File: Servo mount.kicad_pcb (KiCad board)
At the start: 2 copper layers, 80 x 34.1 mm, 40 parts, among them IC1 ATTINY84-SS, J1 SOLDER_PAD, J2 SOLDER_PAD, J3 SOLDER_PAD, J5 SOLDER_PAD, J6 SOLDER_PAD, J7 SOLDER_PAD, J8 SOLDER_PAD, K5 CONN_3, K6 CONN_3, P1 CONN_3X2, Q1 BC847, Q2 BC847, U1 uA78L05, U2 BUZ11

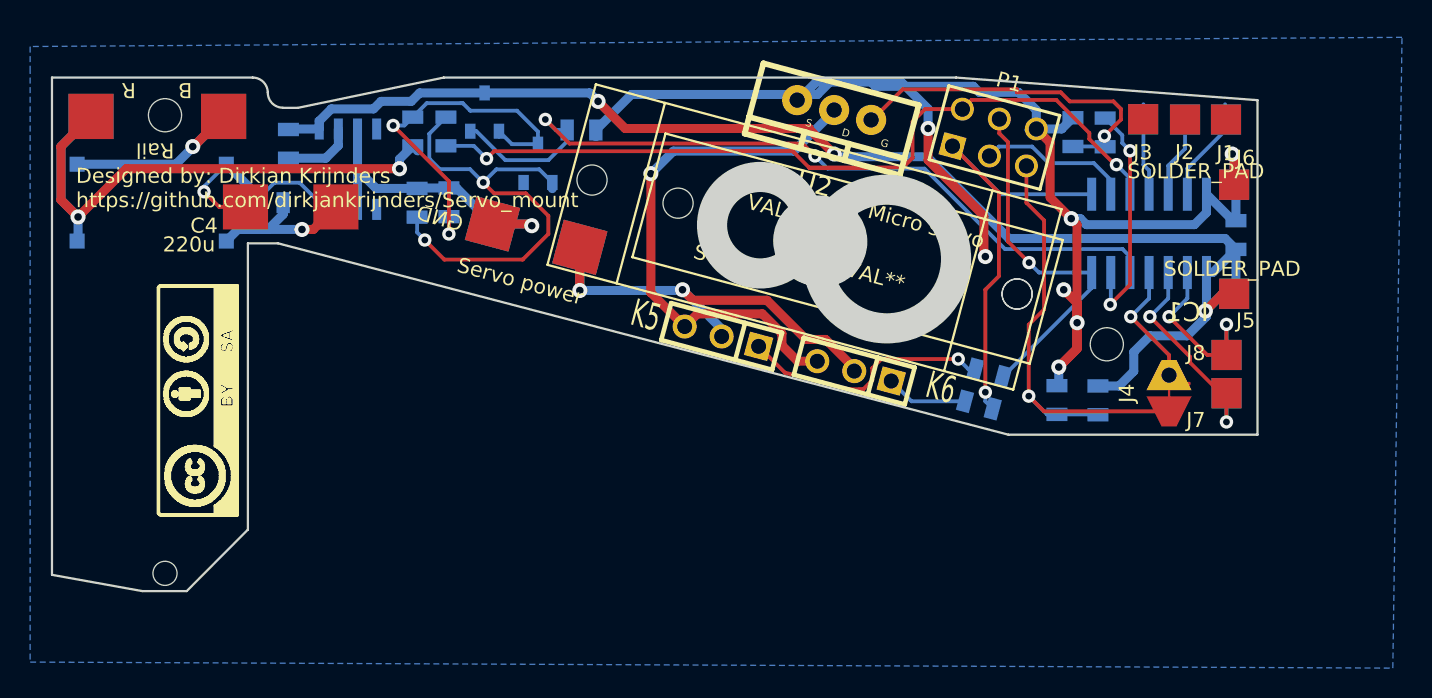
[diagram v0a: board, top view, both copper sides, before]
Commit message: Updates to rev. 3x
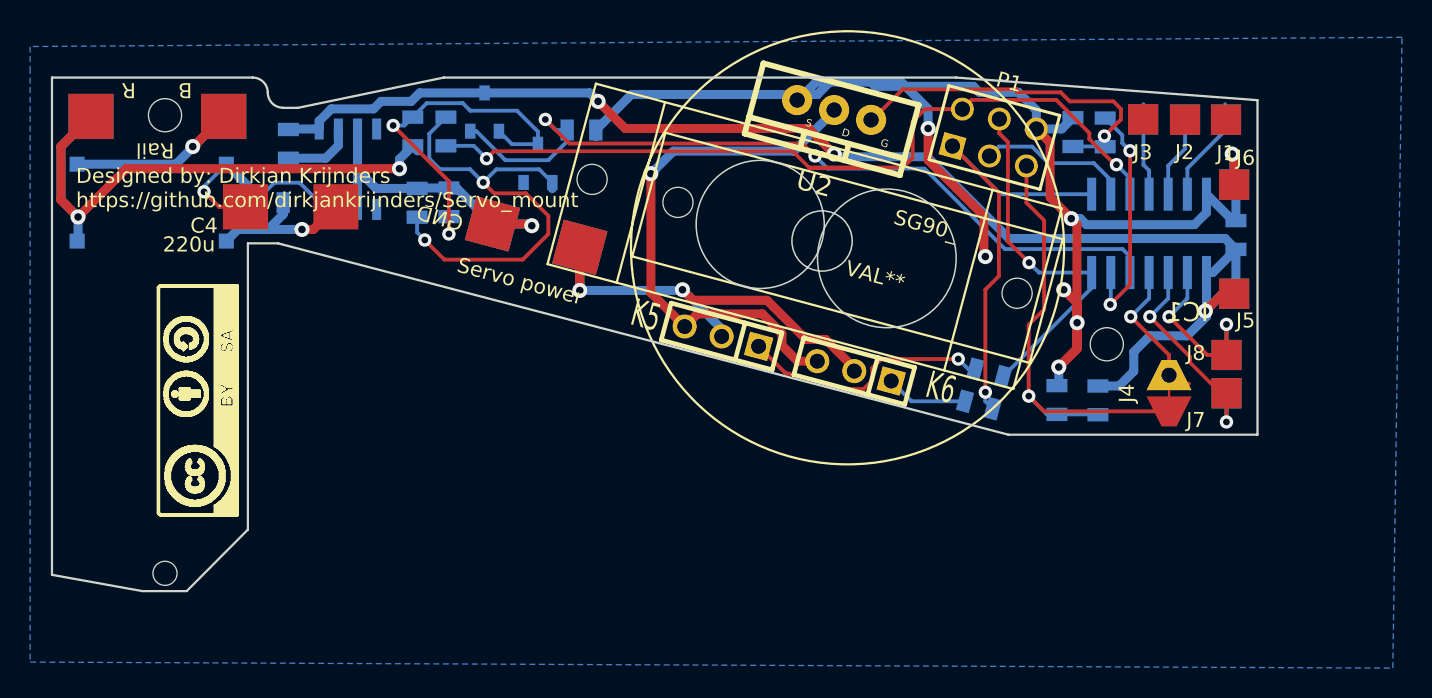
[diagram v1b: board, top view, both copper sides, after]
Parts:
- removed Micro servo: VAL**, Micro_servo
- SG90_: footprint Pyth_servos:Micro_servo_SG90 -> Pyth_servos:Combined_servo
- moved SG90_ 2.94 mm to (152.8, 111.3), turned to 345 degrees
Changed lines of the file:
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@@
     (tracks 380)
     (zones 0)
-    (modules 40)
+    (modules 39)
     (nets 26)
   )
@@
       (net 2 -VAA))
   )
-  (module Micro_servo (layer F.Cu)
-    (at 152.8 111.35 345)
-    (tags HD-1370A)
-    (fp_text reference "Micro servo" (at 4.65 -2.8 345) (layer F.SilkS)
-      (effects (font (size 1 1) (thickness 0.15)))
-    )
-    (fp_text value VAL** (at 2.25 1.3 345) (layer F.SilkS)
-      (effects (font (size 1 1) (thickness 0.15)))
-    )
-    (fp_circle (center -2 0) (end 0 -0.2) (layer Edge.Cuts) (width 2))
-    (fp_circle (center -6 0) (end -3.5 2) (layer Edge.Cuts) (width 2))
-    (fp_line (start 13.65 4.25) (end -13.65 4.25) (layer F.SilkS) (width 0.15))
-    (fp_line (start -13.65 -4.25) (end 13.65 -4.25) (layer F.SilkS) (width 0.15))
-    (fp_line (start 13.65 -4.25) (end 13.65 4.25) (layer F.SilkS) (width 0.15))
-    (fp_line (start -13.65 -4.25) (end -13.65 4.25) (layer F.SilkS) (width 0.15))
-    (pad "" np_thru_hole circle (at -11.65 0 345) (size 2 2) (drill 2) (layers *.Cu *.Mask F.SilkS))
-    (pad "" np_thru_hole circle (at 11.65 0 345) (size 2 2) (drill 2) (layers *.Cu *.Mask F.SilkS))
-  )
   (module solder_jumper_conn (layer F.Cu)
     (at 174.13 120.95 90)
@@
     (pad 1 smd rect (at -0.9525 -1.27 180) (size 0.70104 1.00076) (layers B.Cu B.Paste B.Mask)
       (net 25 "Net-(Q1-Pad1)"))
-    (model smd/SOT23_6.wrl
+    (model smd/smd_transistors/sot23.wrl
       (at (xyz 0 0 0))
-      (scale (xyz 0.11 0.11 0.11))
-      (rotate (xyz 0 0 -180))
+      (scale (xyz 1 1 1))
+      (rotate (xyz 0 0 0))
     )
   )
@@
     (model smd/smd_transistors/sot23.wrl
       (at (xyz 0 0 0))
-      (scale (xyz 0.11 0.11 0.11))
-      (rotate (xyz 0 0 -180))
+      (scale (xyz 1 1 1))
+      (rotate (xyz 0 0 0))
     )
   )
@@
       (net 3 AGND))
   )
-  (module Pyth_servos:Micro_servo_SG90 (layer F.Cu)
-    (at 149.94 110.58 165)
-    (tags SG90)
-    (fp_text reference SG90_ (at 4.65 -2.8 165) (layer F.SilkS)
-      (effects (font (size 1 1) (thickness 0.15)))
-    )
-    (fp_text value VAL** (at 2.25 1.3 165) (layer F.SilkS)
-      (effects (font (size 1 1) (thickness 0.15)))
-    )
-    (fp_line (start 11.25 -6.2) (end 11.25 6.2) (layer F.SilkS) (width 0.15))
-    (fp_line (start -11.25 -6.2) (end -11.25 6.2) (layer F.SilkS) (width 0.15))
-    (fp_circle (center -1.2 0) (end 0.8 -0.2) (layer Edge.Cuts) (width 2))
-    (fp_circle (center -5.65 0) (end -1.05 0) (layer Edge.Cuts) (width 2))
-    (fp_line (start 16 6.2) (end -16 6.2) (layer F.SilkS) (width 0.15))
-    (fp_line (start -16 -6.2) (end 16 -6.2) (layer F.SilkS) (width 0.15))
-    (fp_line (start 16 -6.2) (end 16 6.2) (layer F.SilkS) (width 0.15))
-    (fp_line (start -16 -6.2) (end -16 6.2) (layer F.SilkS) (width 0.15))
-    (pad "" np_thru_hole circle (at -14.6 0 165) (size 2 2) (drill 2) (layers *.Cu *.Mask F.SilkS))
-    (pad "" np_thru_hole circle (at 14.6 0 165) (size 2 2) (drill 2) (layers *.Cu *.Mask F.SilkS))
-    (model ../Pyth_kicad_lib/models/Servo_SG90.wrl
-      (at (xyz 0 0 0))
-      (scale (xyz 1 1 1))
-      (rotate (xyz 0 0 0))
-    )
-  )
   (module Pyth:solder_pad_2mm_fb (layer F.Cu)
     (at 178.448 114.346)
@@
       (effects (font (size 1 1) (thickness 0.15)))
     )
-    (fp_text value SOLDER_PAD (at -0.127 -1.651) (layer F.SilkS)
+    (fp_text value SOLDER_PAD (at -0.127 -1.651) (layer F.SilkS) hide
       (effects (font (size 1 1) (thickness 0.15)))
     )
@@
       (effects (font (size 1 1) (thickness 0.15)))
     )
-    (fp_text value SOLDER_PAD (at -2.54 -0.889) (layer F.SilkS)
+    (fp_text value SOLDER_PAD (at -2.54 -0.889) (layer F.SilkS) hide
       (effects (font (size 1 1) (thickness 0.15)))
     )
@@
       (net 14 "Net-(IC1-Pad2)"))
   )
+  (module Pyth_servos:Combined_servo (layer F.Cu)
+    (at 152.794 111.298 345)
+    (tags HD-1370A)
+    (fp_text reference SG90_ (at 4.65 -2.8 345) (layer F.SilkS)
+      (effects (font (size 1 1) (thickness 0.15)))
+    )
+    (fp_text value VAL** (at 2.25 1.3 345) (layer F.SilkS)
+      (effects (font (size 1 1) (thickness 0.15)))
+    )
+    (fp_circle (center 0 0) (end 12.55 7) (layer F.SilkS) (width 0.15))
+    (fp_line (start 13.65 4.25) (end -13.65 4.25) (layer F.SilkS) (width 0.15))
+    (fp_line (start -13.65 -4.25) (end 13.65 -4.25) (layer F.SilkS) (width 0.15))
+    (fp_line (start 13.65 -4.25) (end 13.65 4.25) (layer F.SilkS) (width 0.15))
+    (fp_line (start -13.65 -4.25) (end -13.65 4.25) (layer F.SilkS) (width 0.15))
+    (fp_circle (center -6 0) (end -1.75 0) (layer Edge.Cuts) (width 0.1))
+    (fp_line (start -14.2 -6.205) (end -14.2 6.195) (layer F.SilkS) (width 0.15))
+    (fp_line (start 8.3 -6.205) (end 8.3 6.195) (layer F.SilkS) (width 0.15))
+    (fp_circle (center -1.75 0) (end -3.75 -0.005) (layer Edge.Cuts) (width 0.1))
+    (fp_circle (center 2.7 0) (end -1.9 -0.005) (layer Edge.Cuts) (width 0.1))
+    (fp_line (start -18.95 6.2) (end 13.05 6.2) (layer F.SilkS) (width 0.15))
+    (fp_line (start 13.05 -6.2) (end -18.95 -6.2) (layer F.SilkS) (width 0.15))
+    (fp_line (start -18.95 -6.2) (end -18.95 6.2) (layer F.SilkS) (width 0.15))
+    (fp_line (start 13.05 -6.2) (end 13.05 6.2) (layer F.SilkS) (width 0.15))
+    (pad "" np_thru_hole circle (at -11.65 0 345) (size 2 2) (drill 2) (layers *.Cu *.Mask F.SilkS))
+    (pad "" np_thru_hole circle (at 11.65 0 345) (size 2 2) (drill 2) (layers *.Cu *.Mask F.SilkS))
+    (pad "" np_thru_hole circle (at -17.55 0 165) (size 2 2) (drill 2) (layers *.Cu *.Mask F.SilkS))
+    (model ../Pyth_kicad_lib/models/Servo_SG90.wrl
+      (at (xyz 0 0 0))
+      (scale (xyz 1 1 1))
+      (rotate (xyz 0 0 0))
+    )
+  )
   (gr_line (start 106 134.08) (end 108.94 134.08) (angle 90) (layer Edge.Cuts) (width 0.15))
